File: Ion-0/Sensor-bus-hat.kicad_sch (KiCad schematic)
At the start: 89 parts, among them J10 Conn_Heater, J11 Conn_01x02, J12 Conn_01x02, J13 Conn_01x04, J6 Coaxial_Small, J7 Conn_01x02, J8 Conn_Heater, J9 Conn_Heater, Q1 IRLML6244, Q2 IRLML6244, Q3 IRLML6244, Q4 IRLML6244, U2 LMT84DCK, U3 BNO085, U4 TCA9617ADGKR, U5 LMT84DCK, U6 MAX-M10M-00B, U7 TPS3850H50DRCR, U8 SN65HVD230, U9 MS860702BA01-50, Y2 9HT10-32.768KBZF-T

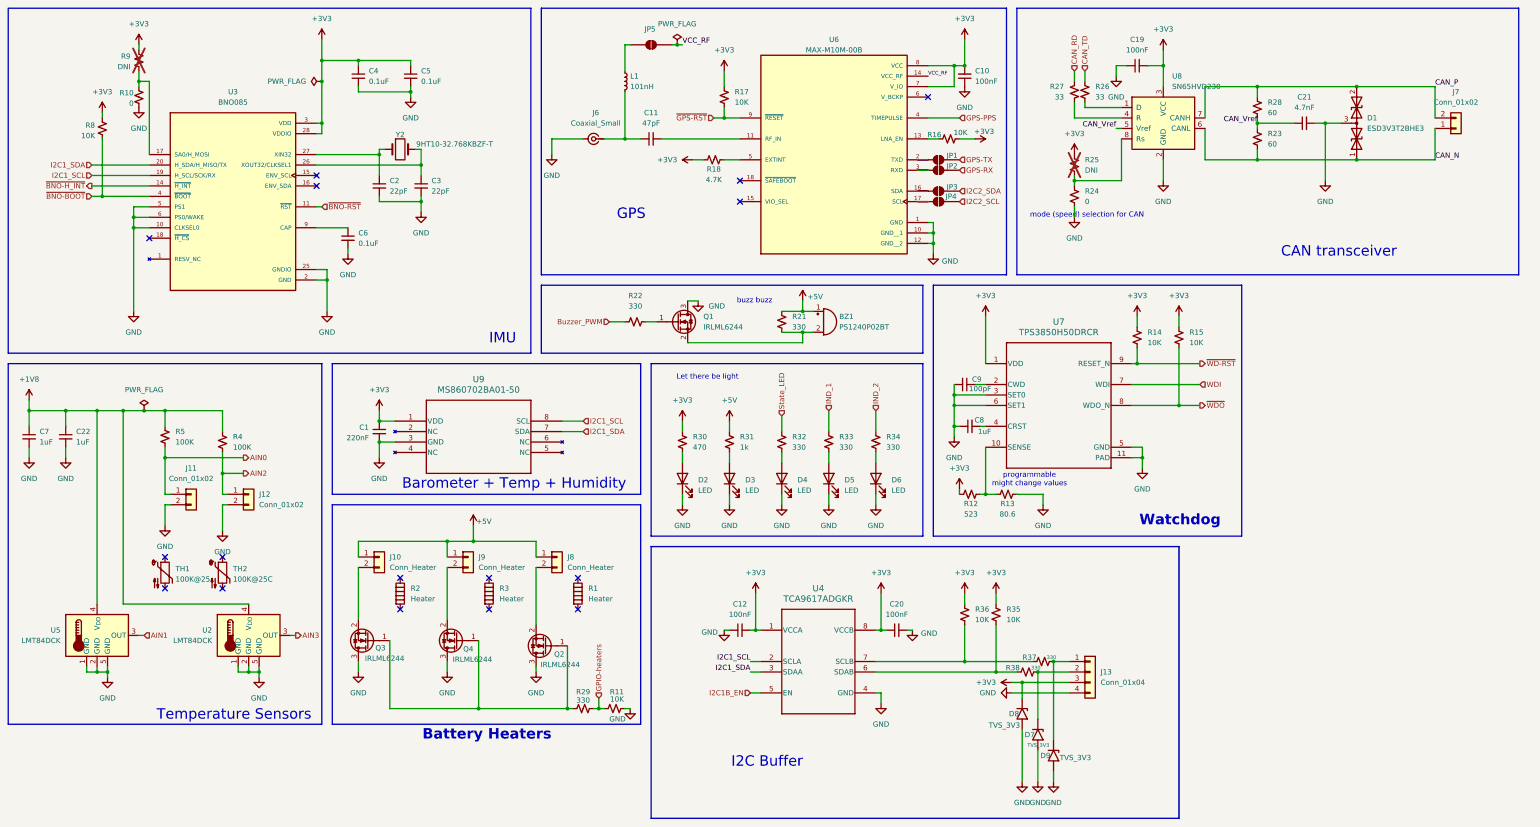
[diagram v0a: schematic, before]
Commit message: restarting layout
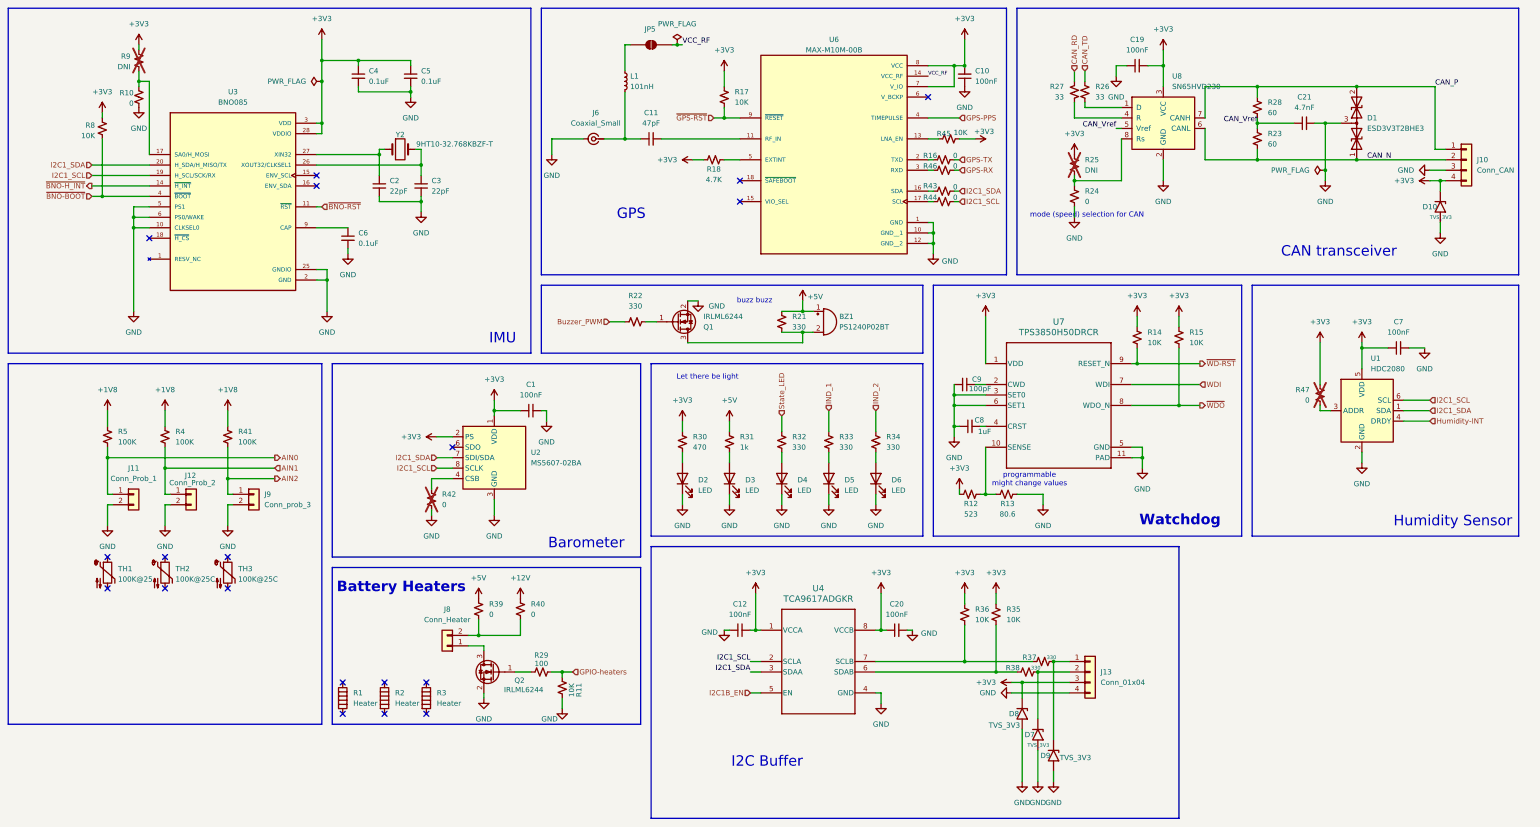
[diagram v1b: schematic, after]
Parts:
- removed C22: 1uF, Capacitor_SMD:C_0603_1608Metric, symbol Device:C_Small
- removed J10: Conn_Heater, Connector_JST:JST_SH_SM02B-SRSS-TB_1x02-1MP_P1.00mm_Horizontal, symbol Connector_Generic:Conn_01x02
- removed J7: Conn_01x02, Connector_JST:JST_SH_SM02B-SRSS-TB_1x02-1MP_P1.00mm_Horizontal, symbol Connector_Generic:Conn_01x02
- removed JP1, JP2, JP3, JP4: SolderJumper_2_Open, Jumper:SolderJumper-2_P1.3mm_Open_TrianglePad1.0x1.5mm, symbol Jumper:SolderJumper_2_Open
- removed Q3, Q4: IRLML6244, Package_TO_SOT_SMD:SOT-23, symbol Transistor_FET:IRLML6244
- removed U2, U5: LMT84DCK, Package_TO_SOT_SMD:SOT-353_SC-70-5, symbol Sensor_Temperature:LMT84DCK
- removed U9: MS860702BA01-50, 1_Ion:MS860702BA01-50_TEC, symbol 1_ion_library:MS860702BA01-50
- added D10: TVS_3V3, Diode_SMD:D_0402_1005Metric_Pad0.77x0.64mm_HandSolder, symbol Diode:SM6T33A
- added J10: Conn_CAN, Connector_JST:JST_SH_BM04B-SRSS-TB_1x04-1MP_P1.00mm_Vertical, symbol Connector_Generic:Conn_01x04
- added R39, R40: 0, Resistor_SMD:R_1206_3216Metric, symbol Device:R_Small_US
- added R41: 100K, Resistor_SMD:R_0603_1608Metric_Pad0.98x0.95mm_HandSolder, symbol Device:R_Small_US
- added R42, R47: 0, symbol Device:R_Small_US
- added R43, R44, R45, R46: 0, Resistor_SMD:R_0603_1608Metric_Pad0.98x0.95mm_HandSolder, symbol Device:R_Small_US
- added TH3: 100K@25C, symbol Device:Thermistor_NTC
- added U1: HDC2080, Sensor_Humidity:Texas_S-PWSON-N6-HDC2080, symbol Sensor_Humidity:HDC2080
- added U2: MS5607-02BA, Package_LGA:LGA-8_3x5mm_P1.25mm, symbol Sensor_Pressure:MS5607-02BA
- C1: value 220nF -> 100nF
- C7: value 1uF -> 100nF
- J11: value Conn_01x02 -> Conn_Prob_1; footprint Connector_JST:JST_SH_SM02B-SRSS-TB_1x02-1MP_P1.00mm_Horizontal -> TerminalBlock:TerminalBlock_Xinya_XY308-2.54-2P_1x02_P2.54mm_Horizontal
- J12: value Conn_01x02 -> Conn_Prob_2; footprint Connector_JST:JST_SH_SM02B-SRSS-TB_1x02-1MP_P1.00mm_Horizontal -> TerminalBlock:TerminalBlock_Xinya_XY308-2.54-2P_1x02_P2.54mm_Horizontal
- J6: footprint Connector_Coaxial:SMA_Samtec_SMA-J-P-H-ST-EM1_EdgeMount -> Connector_Coaxial:U.FL_Molex_MCRF_73412-0110_Vertical
- J8: footprint Connector_JST:JST_SH_SM02B-SRSS-TB_1x02-1MP_P1.00mm_Horizontal -> TerminalBlock:TerminalBlock_Xinya_XY308-2.54-2P_1x02_P2.54mm_Horizontal
- J9: value Conn_Heater -> Conn_prob_3; footprint Connector_JST:JST_SH_SM02B-SRSS-TB_1x02-1MP_P1.00mm_Horizontal -> TerminalBlock:TerminalBlock_Xinya_XY308-2.54-2P_1x02_P2.54mm_Horizontal
- R29: value 330 -> 100
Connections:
- net +1V8: now also R41.1; no longer C7.1
- net +3V3: now also C7.1, D10.1 (A1), J10.4 (Pin_4), R47.1, U1.5 (VDD), U2.1 (VDD), U2.2 (PS)
- net +5V: now also R39.1; no longer J8.1 (Pin_1), J9.1 (Pin_1)
- net AIN1: now also J12.1 (Pin_1), R4.2
- net AIN2: now also J9.1 (Pin_1), R41.2; no longer J12.1 (Pin_1), R4.2
- net CAN_N: now also J10.2 (Pin_2)
- net CAN_P: now also J10.1 (Pin_1)
- net GND: now also J9.2 (Pin_2), Q1.2 (S), Q2.2 (S), D10.2 (A2), J10.3 (Pin_3), R42.2, U1.2 (GND), U2.3 (GND); no longer Q1.3 (D), Q2.3 (D)
- net GPS-RX: now also R46.2
- net GPS-TX: now also R45.1
- net I2C1_SCL: now also R44.1, U1.6 (SCL), U2.8 (SCLK)
- net I2C1_SDA: now also R43.1, U1.1 (SDA), U2.7 (SDI/SDA)
- net at U6.3 (RXD): now also R46.1
- net at BZ1.2 (-), R21.2: now also Q1.3 (D); no longer Q1.2 (S)
- net at U6.16 (SDA): now also R43.2
- net at U6.17 (SCL): now also R44.2
- net at U6.2 (TXD): now also R45.2
- net at J8.2 (Pin_2): now also R39.2, R40.2; no longer Q2.2 (S)
- new net: R42.1, U2.4 (CSB), U2.5 (CSB)
- new net: R47.2, U1.3 (ADDR)
- new net: J8.1 (Pin_1), Q2.3 (D)
- new net +12V: R40.1
- new net Humidity-INT: U1.4 (DRDY)
- no-connect marks 16 -> 19
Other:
- note added: "Barometer"
- note added: "Humidity Sensor"
- note removed: "Barometer + Temp + Humidity"
- note removed: "Temperature Sensors"
- moved on the sheet: J11, J12, J8, Q2, R1, R11, R2, R29, R3, R4, R5, TH1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
